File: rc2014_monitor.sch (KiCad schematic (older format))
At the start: 24 parts, among them J1 RC2014Pro, J2 Conn_01x23, SW1 SW_Coded_Octal, U1 74LS138, U2 74LS151, U3 74HCT244, U4 74HCT244, U5 74HCT244

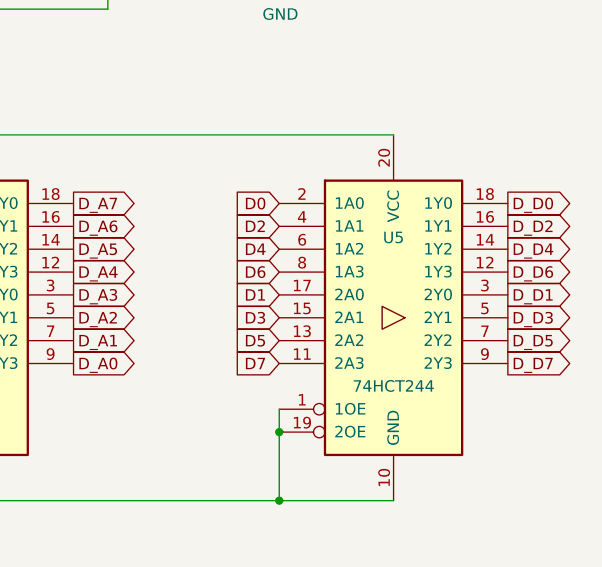
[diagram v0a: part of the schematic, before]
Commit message: started adding traces
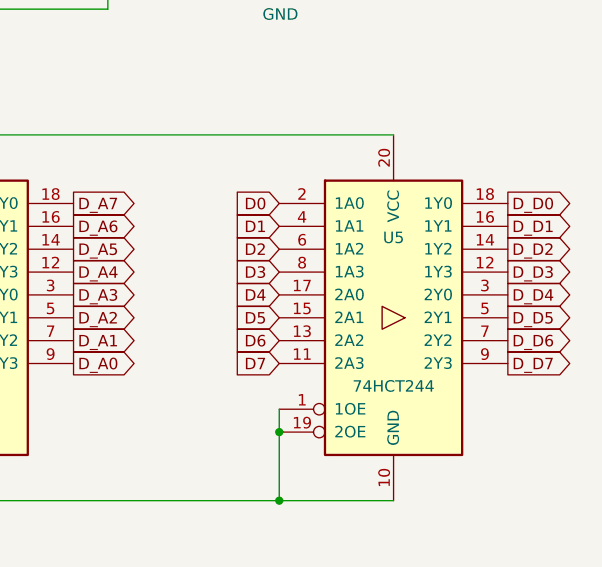
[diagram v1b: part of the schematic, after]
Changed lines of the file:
@@
 Text GLabel 8850 3650 2    50   Output ~ 0
 D_A4
-Text GLabel 9750 3850 0    50   Input ~ 0
+Text GLabel 9750 3650 0    50   Input ~ 0
 D3
+Text GLabel 9750 3550 0    50   Input ~ 0
+D2
 Text GLabel 9750 3450 0    50   Input ~ 0
-D2
-Text GLabel 9750 3750 0    50   Input ~ 0
 D1
 Text GLabel 9750 3350 0    50   Input ~ 0
@@
 Text GLabel 9750 4050 0    50   Input ~ 0
 D7
-Text GLabel 9750 3650 0    50   Input ~ 0
+Text GLabel 9750 3950 0    50   Input ~ 0
 D6
-Text GLabel 9750 3950 0    50   Input ~ 0
+Text GLabel 9750 3850 0    50   Input ~ 0
 D5
-Text GLabel 9750 3550 0    50   Input ~ 0
+Text GLabel 9750 3750 0    50   Input ~ 0
 D4
-Text GLabel 10750 3850 2    50   Output ~ 0
+Text GLabel 10750 3650 2    50   Output ~ 0
 D_D3
 Text GLabel 10750 3450 2    50   Output ~ 0
-D_D2
-Text GLabel 10750 3750 2    50   Output ~ 0
 D_D1
 Text GLabel 10750 3350 2    50   Output ~ 0
@@
 Text GLabel 10750 4050 2    50   Output ~ 0
 D_D7
-Text GLabel 10750 3650 2    50   Output ~ 0
+Text GLabel 10750 3950 2    50   Output ~ 0
 D_D6
-Text GLabel 10750 3950 2    50   Output ~ 0
+Text GLabel 10750 3850 2    50   Output ~ 0
 D_D5
-Text GLabel 10750 3550 2    50   Output ~ 0
+Text GLabel 10750 3750 2    50   Output ~ 0
 D_D4
 $Comp
@@
 NoConn ~ 1600 5700
 NoConn ~ 1600 5800
+Text GLabel 10750 3550 2    50   Output ~ 0
+D_D2
 $EndSCHEMATC

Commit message: finished traces and silkscreens
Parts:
- C1, C2, C4, C5: MouserPN (none) -> 75-1C10Z5U104M050R
- DISP0, DISP1, DISP2, DISP3, DISP4, DISP5: symbol Display_Character:TIL311 -> rc2014_monitor-rescue:TIL311-Display_Character
- LED1, LED2, LED3, LED4, LED5: MouserPN (none) -> 755-SML-H12U8TT86C
- RN1: Mouser PN 652-4607X-1LF-270 -> (none); MouserPN (none) -> 652-4607X-1LF-270
- SW1: footprint Button_Switch_SMD:Nidec_Copal_SH-7010B -> Connector_PinHeader_2.54mm:PinHeader_2x03_P2.54mm_Vertical; symbol Switch:SW_Coded_Octal -> rc2014_monitor-rescue:SW_Coded_Octal-Switch; Mouser PN 706-94HBB08RAT -> (none); MouserPN (none) -> 706-94HBB08RAT
- U1: MouserPN (none) -> 595-SN74LS138N
- U2: MouserPN (none) -> 595-SN74LS151N
- U3, U4, U5: MouserPN (none) -> 595-SN74HCT244N
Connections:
- wire segments 120 -> 118
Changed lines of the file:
@@
 $EndDescr
 $Comp
-L Display_Character:TIL311 DISP5
+L rc2014_monitor-rescue:TIL311-Display_Character DISP5
 U 1 1 5CB4BA92
 P 1950 1500
@@
 $EndComp
 $Comp
-L Display_Character:TIL311 DISP4
+L rc2014_monitor-rescue:TIL311-Display_Character DISP4
 U 1 1 5CB4CB07
 P 3500 1500
@@
 $EndComp
 $Comp
-L Display_Character:TIL311 DISP3
+L rc2014_monitor-rescue:TIL311-Display_Character DISP3
 U 1 1 5CB4D9E8
 P 5050 1500
@@
 $EndComp
 $Comp
-L Display_Character:TIL311 DISP2
+L rc2014_monitor-rescue:TIL311-Display_Character DISP2
 U 1 1 5CB570C9
 P 6600 1500
@@
 $EndComp
 $Comp
-L Display_Character:TIL311 DISP0
+L rc2014_monitor-rescue:TIL311-Display_Character DISP0
 U 1 1 5CB570D5
 P 9750 1500
@@
 F 1 "74HCT244" H 6450 3550 50  0000 C CNN
 F 2 "Package_DIP:DIP-20_W7.62mm_Socket_LongPads" H 6450 3850 50  0001 C CNN
-F 3 "https://assets.nexperia.com/documents/data-sheet/74HC_HCT244.pdf" H 6450 3850 50  0001 C CNN
+F 3 "http://www.ti.com/lit/ds/symlink/sn74hct244.pdf" H 6450 3850 50  0001 C CNN
+F 4 "595-SN74HCT244N" H 0   0   50  0001 C CNN "MouserPN"
 	1    6450 3850
 	1    0    0    -1
@@
 F 1 "74HCT244" H 8350 3550 50  0000 C CNN
 F 2 "Package_DIP:DIP-20_W7.62mm_Socket_LongPads" H 8350 3850 50  0001 C CNN
-F 3 "https://assets.nexperia.com/documents/data-sheet/74HC_HCT244.pdf" H 8350 3850 50  0001 C CNN
+F 3 "http://www.ti.com/lit/ds/symlink/sn74hct244.pdf" H 8350 3850 50  0001 C CNN
+F 4 "595-SN74HCT244N" H 0   0   50  0001 C CNN "MouserPN"
 	1    8350 3850
 	1    0    0    -1
@@
 F 1 "WR" H 4750 3550 50  0000 C CNN
 F 2 "LED_SMD:LED_0805_2012Metric_Pad1.15x1.40mm_HandSolder" V 4850 3500 50  0001 C CNN
-F 3 "~" V 4850 3500 50  0001 C CNN
+F 3 "https://www.mouser.com/datasheet/2/348/sml-h1(c)-e-1508182.pdf" V 4850 3500 50  0001 C CNN
+F 4 "755-SML-H12U8TT86C" H 0   0   50  0001 C CNN "MouserPN"
 	1    4850 3500
 	1    0    0    -1
@@
 F 1 "RD" H 4750 3650 50  0000 C CNN
 F 2 "LED_SMD:LED_0805_2012Metric_Pad1.15x1.40mm_HandSolder" V 4850 3600 50  0001 C CNN
-F 3 "~" V 4850 3600 50  0001 C CNN
+F 3 "https://www.mouser.com/datasheet/2/348/sml-h1(c)-e-1508182.pdf" V 4850 3600 50  0001 C CNN
+F 4 "755-SML-H12U8TT86C" H 0   0   50  0001 C CNN "MouserPN"
 	1    4850 3600
 	1    0    0    -1
@@
 F 1 "IORQ" H 4750 3750 50  0000 C CNN
 F 2 "LED_SMD:LED_0805_2012Metric_Pad1.15x1.40mm_HandSolder" V 4850 3700 50  0001 C CNN
-F 3 "~" V 4850 3700 50  0001 C CNN
+F 3 "https://www.mouser.com/datasheet/2/348/sml-h1(c)-e-1508182.pdf" V 4850 3700 50  0001 C CNN
+F 4 "755-SML-H12U8TT86C" H 0   0   50  0001 C CNN "MouserPN"
 	1    4850 3700
 	1    0    0    -1
@@
 F 1 "MREQ" H 4750 3850 50  0000 C CNN
 F 2 "LED_SMD:LED_0805_2012Metric_Pad1.15x1.40mm_HandSolder" V 4850 3800 50  0001 C CNN
-F 3 "~" V 4850 3800 50  0001 C CNN
+F 3 "https://www.mouser.com/datasheet/2/348/sml-h1(c)-e-1508182.pdf" V 4850 3800 50  0001 C CNN
+F 4 "755-SML-H12U8TT86C" H 0   0   50  0001 C CNN "MouserPN"
 	1    4850 3800
 	1    0    0    -1
@@
 F 1 "M1" H 4750 3950 50  0000 C CNN
 F 2 "LED_SMD:LED_0805_2012Metric_Pad1.15x1.40mm_HandSolder" V 4850 3900 50  0001 C CNN
-F 3 "~" V 4850 3900 50  0001 C CNN
+F 3 "https://www.mouser.com/datasheet/2/348/sml-h1(c)-e-1508182.pdf" V 4850 3900 50  0001 C CNN
+F 4 "755-SML-H12U8TT86C" H 0   0   50  0001 C CNN "MouserPN"
 	1    4850 3900
 	1    0    0    -1
@@
 F 1 "100nf" H 8515 5505 50  0000 L CNN
 F 2 "Capacitor_THT:C_Disc_D3.0mm_W1.6mm_P2.50mm" H 8438 5400 50  0001 C CNN
-F 3 "~" H 8400 5550 50  0001 C CNN
+F 3 "https://www.mouser.com/datasheet/2/427/Sprague%201C-3C%20MLC%20leaded%20capacitors%202000-1211470.pdf" H 8400 5550 50  0001 C CNN
+F 4 "75-1C10Z5U104M050R" H 0   0   50  0001 C CNN "MouserPN"
 	1    8400 5550
 	1    0    0    -1
@@
 F 1 "100nf" H 8065 5505 50  0000 L CNN
 F 2 "Capacitor_THT:C_Disc_D3.0mm_W1.6mm_P2.50mm" H 7988 5400 50  0001 C CNN
-F 3 "~" H 7950 5550 50  0001 C CNN
+F 3 "https://www.mouser.com/datasheet/2/427/Sprague%201C-3C%20MLC%20leaded%20capacitors%202000-1211470.pdf" H 7950 5550 50  0001 C CNN
+F 4 "75-1C10Z5U104M050R" H 0   0   50  0001 C CNN "MouserPN"
 	1    7950 5550
 	1    0    0    -1
@@
 F 2 "Package_DIP:DIP-16_W7.62mm_Socket_LongPads" H 4000 5950 50  0001 C CNN
 F 3 "http://www.ti.com/lit/gpn/sn74LS151" H 4000 5950 50  0001 C CNN
+F 4 "595-SN74LS151N" H 0   0   50  0001 C CNN "MouserPN"
 	1    4000 5950
 	1    0    0    -1
@@
 	1    0    0    -1
 $EndComp
-$Comp
-L Switch:SW_Coded_Octal SW?
-U 1 1 5CA7C108
-P 2400 3550
-AR Path="/5CB5AB00/5CB63856/5CA7C108" Ref="SW?"  Part="1"
-AR Path="/5CA7C108" Ref="SW1"  Part="1"
-F 0 "SW1" H 2532 4025 50  0000 C CNN
-F 1 "SW_Coded_Octal" H 2532 3934 50  0000 C CNN
-F 2 "Button_Switch_SMD:Nidec_Copal_SH-7010B" H 2375 3575 50  0001 C CNN
-F 3 "https://www.mouser.com/datasheet/2/626/DIP_Series_94H-334494.pdf" H 2375 3575 50  0001 C CNN
-F 4 "706-94HBB08RAT" H 2500 3150 50  0001 C CNN "Mouser PN"
-	1    2400 3550
-	1    0    0    -1
-$EndComp
 NoConn ~ 4500 4200
 NoConn ~ 4500 4100
@@
 F 2 "Package_DIP:DIP-16_W7.62mm_Socket_LongPads" H 4000 3800 50  0001 C CNN
 F 3 "http://www.ti.com/lit/gpn/sn74LS138" H 4000 3800 50  0001 C CNN
+F 4 "595-SN74LS138N" H 0   0   50  0001 C CNN "MouserPN"
 	1    4000 3800
 	1    0    0    -1
@@
 F 1 "100nf" H 9515 5505 50  0000 L CNN
 F 2 "Capacitor_THT:C_Disc_D3.0mm_W1.6mm_P2.50mm" H 9438 5400 50  0001 C CNN
-F 3 "~" H 9400 5550 50  0001 C CNN
+F 3 "https://www.mouser.com/datasheet/2/427/Sprague%201C-3C%20MLC%20leaded%20capacitors%202000-1211470.pdf" H 9400 5550 50  0001 C CNN
+F 4 "75-1C10Z5U104M050R" H 0   0   50  0001 C CNN "MouserPN"
 	1    9400 5550
 	1    0    0    -1
@@
 F 1 "100nf" H 10015 5505 50  0000 L CNN
 F 2 "Capacitor_THT:C_Disc_D3.0mm_W1.6mm_P2.50mm" H 9938 5400 50  0001 C CNN
-F 3 "~" H 9900 5550 50  0001 C CNN
+F 3 "https://www.mouser.com/datasheet/2/427/Sprague%201C-3C%20MLC%20leaded%20capacitors%202000-1211470.pdf" H 9900 5550 50  0001 C CNN
+F 4 "75-1C10Z5U104M050R" H 0   0   50  0001 C CNN "MouserPN"
 	1    9900 5550
 	1    0    0    -1
@@
 Wire Wire Line
 	3000 3600 3500 3600
-Connection ~ 2900 3500
 Connection ~ 4000 4500
 Connection ~ 9400 5400
@@
 Connection ~ 8200 800
 $Comp
-L Display_Character:TIL311 DISP1
+L rc2014_monitor-rescue:TIL311-Display_Character DISP1
 U 1 1 5CB570CF
 P 8100 1500
@@
 F 1 "74HCT244" H 10250 3550 50  0000 C CNN
 F 2 "Package_DIP:DIP-20_W7.62mm_Socket_LongPads" H 10250 3850 50  0001 C CNN
-F 3 "https://assets.nexperia.com/documents/data-sheet/74HC_HCT244.pdf" H 10250 3850 50  0001 C CNN
+F 3 "http://www.ti.com/lit/ds/symlink/sn74hct244.pdf" H 10250 3850 50  0001 C CNN
+F 4 "595-SN74HCT244N" H 0   0   50  0001 C CNN "MouserPN"
 	1    10250 3850
 	1    0    0    -1
@@
 Text GLabel 1350 1550 0    50   Input ~ 0
 D_A12
-Wire Wire Line
-	2900 3500 2900 3600
 Wire Wire Line
 	3500 5850 3350 5850
@@
 F 2 "Resistor_THT:R_Array_SIP7" V 5725 3800 50  0001 C CNN
 F 3 "https://www.mouser.com/datasheet/2/54/600x-776645.pdf" H 5350 3800 50  0001 C CNN
-F 4 "652-4607X-1LF-270" V 5350 3800 50  0001 C CNN "Mouser PN"
+F 4 "652-4607X-1LF-270" V 5350 3800 50  0001 C CNN "MouserPN"
 	1    5350 3800
 	0    1    1    0
 $EndComp
-Connection ~ 2900 3600
-Wire Wire Line
-	2900 3600 2900 3700
-Connection ~ 2900 3700
-Wire Wire Line
-	2900 3700 2900 6450
 Wire Wire Line
 	5650 3100 5650 3500
@@
 Text GLabel 10750 3550 2    50   Output ~ 0
 D_D2
+Wire Wire Line
+	2900 3500 2900 6450
+Connection ~ 2900 3500
+$Comp
+L rc2014_monitor-rescue:SW_Coded_Octal-Switch SW?
+U 1 1 5CA7C108
+P 2400 3550
+AR Path="/5CB5AB00/5CB63856/5CA7C108" Ref="SW?"  Part="1"
+AR Path="/5CA7C108" Ref="SW1"  Part="1"
+F 0 "SW1" H 2532 4025 50  0000 C CNN
+F 1 "SW_Coded_Octal" H 2532 3934 50  0000 C CNN
+F 2 "Connector_PinHeader_2.54mm:PinHeader_2x03_P2.54mm_Vertical" H 2375 3575 50  0001 C CNN
+F 3 "https://www.mouser.com/datasheet/2/626/DIP_Series_94H-334494.pdf" H 2375 3575 50  0001 C CNN
+F 4 "706-94HBB08RAT" H 2500 3150 50  0001 C CNN "MouserPN"
+	1    2400 3550
+	1    0    0    -1
+$EndComp
 $EndSCHEMATC

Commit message: updated boms
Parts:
- C1, C2, C4, C5: MFR (none) -> Vishay/Sprague; MPN (none) -> 1C10Z5U104M050R; SPN (none) -> 75-1C10Z5U104M050R; SPR (none) -> Mouser; SPURL (none) -> -
- DISP0, DISP1, DISP2, DISP3, DISP4, DISP5, J1, J2, SW1: MFR (none) -> -; MPN (none) -> -; SPN (none) -> -; SPR (none) -> -; SPURL (none) -> -
- LED1: value WR -> SMD Red 620nm 40mcd 2.2V; 20mA; MFR (none) -> ROHM Semiconductor; MPN (none) -> SML-H12U8TT86C; SPN (none) -> 755-SML-H12U8TT86C; SPR (none) -> Mouser; SPURL (none) -> -
- LED2: value RD -> SMD Red 620nm 40mcd 2.2V; 20mA; MFR (none) -> ROHM Semiconductor; MPN (none) -> SML-H12U8TT86C; SPN (none) -> 755-SML-H12U8TT86C; SPR (none) -> Mouser; SPURL (none) -> -
- LED3: value IORQ -> SMD Red 620nm 40mcd 2.2V; 20mA; MFR (none) -> ROHM Semiconductor; MPN (none) -> SML-H12U8TT86C; SPN (none) -> 755-SML-H12U8TT86C; SPR (none) -> Mouser; SPURL (none) -> -
- LED4: value MREQ -> SMD Red 620nm 40mcd 2.2V; 20mA; MFR (none) -> ROHM Semiconductor; MPN (none) -> SML-H12U8TT86C; SPN (none) -> 755-SML-H12U8TT86C; SPR (none) -> Mouser; SPURL (none) -> -
- LED5: value M1 -> SMD Red 620nm 40mcd 2.2V; 20mA; MFR (none) -> ROHM Semiconductor; MPN (none) -> SML-H12U8TT86C; SPN (none) -> 755-SML-H12U8TT86C; SPR (none) -> Mouser; SPURL (none) -> -
- RN1: MFR (none) -> Bourns; MPN (none) -> 4607X-101-271LF; SPN (none) -> 652-4607X-1LF-270; SPR (none) -> Mouser; SPURL (none) -> -
- U1, U2: MFR (none) -> Texas Instruments; MPN (none) -> SN74LS138N; SPN (none) -> 595-SN74LS138N; SPR (none) -> Mouser; SPURL (none) -> -
- U3, U4, U5: MFR (none) -> Texas Instruments; MPN (none) -> SN74HCT244N; SPN (none) -> 595-SN74HCT244N; SPR (none) -> Mouser; SPURL (none) -> -
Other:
- note added: "IORQ"
- note added: "M1"
- note added: "MREQ"
- note added: "RD"
- note added: "WR"

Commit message: more appropriate latch options
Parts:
- removed C1, C2, C4, C5: 100nf, Capacitor_THT:C_Disc_D3.0mm_W1.6mm_P2.50mm, symbol Device:C
- removed SW1: SW_Coded_Octal, Connector_PinHeader_2.54mm:PinHeader_2x03_P2.54mm_Vertical, symbol rc2014_monitor-rescue:SW_Coded_Octal-Switch
- removed U1: 74LS138, Package_DIP:DIP-16_W7.62mm_Socket_LongPads, symbol 74xx:74LS138
- removed U2: 74LS151, Package_DIP:DIP-16_W7.62mm_Socket_LongPads, symbol 74xx:74LS151
- added D1: Schottky Diodes & Rectifiers 40V Vr; 6A, Package_TO_SOT_SMD:TO-252-3_TabPin2, symbol Device:D_Schottky_x2_KCom_AKA
- added J3: USB_B_Micro, Connector_USB:USB_Micro-B_Amphenol_10103594-0001LF_Horizontal, symbol Connector:USB_B_Micro
- added SW1: SW_Coded_Octal-8, Button_Switch_THT:Nidec_Copal_SH-7010C, symbol Switch:SW_Coded_Octal-8
- added U1: 74HCT138, Package_DIP:DIP-16_W7.62mm_LongPads, symbol 74xx:74HCT138
- added U2: 74HCT151, Package_DIP:DIP-16_W7.62mm_LongPads, symbol 74xx:74HCT151
- added U6: 74HCT32, symbol 74xx:74HCT32
- J2: value Conn_01x23 -> Conn_01x10; footprint Connector_PinHeader_2.54mm:PinHeader_1x23_P2.54mm_Vertical -> Connector_PinHeader_2.54mm:PinHeader_1x10_P2.54mm_Vertical; symbol Connector_Generic:Conn_01x23 -> Connector_Generic:Conn_01x10
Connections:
- net labels added: IO_RD, IO_WR, M_RD, M_WR
- wire segments 118 -> 123
- no-connect marks 46 -> 36
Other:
- note added: "IO_RD\n"
- note added: "IO_WR"
- note added: "MR_RD"
- note added: "MR_WR"
- note removed: "IORQ"
- note removed: "MREQ"
- note removed: "RD"
- note removed: "WR"

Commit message: Added io_rd/wr,mem_rd/wr for latch options
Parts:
- removed J2: Conn_01x10, Connector_PinHeader_2.54mm:PinHeader_1x10_P2.54mm_Vertical, symbol Connector_Generic:Conn_01x10
- SW1: symbol Switch:SW_Coded_Octal-8 -> rc2014_monitor-rescue:SW_Coded_Octal-8-Switch
- U1: symbol 74xx:74HCT138 -> rc2014_monitor-rescue:74HCT138-74xx
- U2: symbol 74xx:74HCT151 -> rc2014_monitor-rescue:74HCT151-74xx
- U6: footprint (none) -> Package_DIP:DIP-14_W7.62mm_LongPads; symbol 74xx:74HCT32 -> rc2014_monitor-rescue:74HCT32-74xx
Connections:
- no-connect marks 36 -> 28
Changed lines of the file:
@@
-$EndComp
-$Comp
-L Connector_Generic:Conn_01x10 J?
-U 1 1 5CA62B20
-P 1400 5300
-AR Path="/5CB5AB00/5CA62B20" Ref="J?"  Part="1"
-AR Path="/5CA62B20" Ref="J2"  Part="1"
-F 0 "J2" H 1400 5950 50  0000 C CNN
-F 1 "Conn_01x10" H 1350 5850 50  0000 C CNN
-F 2 "Connector_PinHeader_2.54mm:PinHeader_1x10_P2.54mm_Vertical" H 1400 5300 50  0001 C CNN
-F 3 "~" H 1400 5300 50  0001 C CNN
-F 4 "-" H 0   -700 50  0001 C CNN "MFR"
-F 5 "-" H 0   -700 50  0001 C CNN "MPN"
-F 6 "-" H 0   -700 50  0001 C CNN "SPR"
-F 7 "-" H 0   -700 50  0001 C CNN "SPN"
-F 8 "-" H 0   -700 50  0001 C CNN "SPURL"
-	1    1400 5300
-	-1   0    0    -1
 $EndComp
 $Comp
@@
 $EndComp
 $Comp
-L power:+5V #PWR0109
-U 1 1 5CAA9BF0
-P 5950 700
-AR Path="/5CAA9BF0" Ref="#PWR0109"  Part="1"
-AR Path="/5CB63856/5CAA9BF0" Ref="#PWR?"  Part="1"
-AR Path="/5CB5AB00/5CB63856/5CAA9BF0" Ref="#PWR?"  Part="1"
-F 0 "#PWR0109" H 5950 550 50  0001 C CNN
-F 1 "+5V" H 5965 873 50  0000 C CNN
-F 2 "" H 5950 700 50  0001 C CNN
-F 3 "" H 5950 700 50  0001 C CNN
-	1    5950 700
-	1    0    0    -1
-$EndComp
-$Comp
 L power:GND #PWR0110
 U 1 1 5CAAC638
@@
 	0    1    1    0
 $EndComp
-Text GLabel 1600 4900 2    50   Output ~ 0
-GND
 Text GLabel 1000 5900 2    50   Output ~ 0
 D0
@@
 Text GLabel 1000 3800 2    50   Output ~ 0
 A10
-Text GLabel 1600 5000 2    50   Output ~ 0
-5V
 Text Notes 600  3000 0    50   ~ 0
 RC2014 Pro Bus
@@
 Text GLabel 10750 3550 2    50   Output ~ 0
 D_D2
-Wire Notes Line
-	550  2850 2050 2850
-Wire Notes Line
-	2050 2850 2050 7400
-Wire Notes Line
-	2050 7400 550  7400
-Wire Notes Line
-	550  7400 550  2850
 Wire Wire Line
 	8350 3050 10250 3050
@@
 	9650 800  9850 800
 Wire Wire Line
-	5950 700  5950 800
+	5850 700  5850 800
 Wire Wire Line
 	1350 1900 1350 2200
@@
 	6000 2200 6600 2200
 Wire Wire Line
-	5950 800  6500 800
-Wire Wire Line
 	9150 1750 9000 1750
 Wire Wire Line
@@
 	3600 800  4950 800
 Wire Wire Line
-	5150 800  5950 800
+	5150 800  5850 800
 Wire Wire Line
 	2050 800  3400 800
@@
 Connection ~ 2750 2500
 Connection ~ 4950 800
-Connection ~ 5950 800
 Connection ~ 3400 800
 Connection ~ 3350 5950
@@
 NoConn ~ 1000 5300
 NoConn ~ 1000 5400
-NoConn ~ 1600 5100
-NoConn ~ 1600 5200
-NoConn ~ 1600 5300
-NoConn ~ 1600 5400
-NoConn ~ 1600 5500
-NoConn ~ 1600 5600
-NoConn ~ 1600 5700
-NoConn ~ 1600 5800
 Text Notes 4550 3500 0    50   ~ 0
 IO_RD\n
@@
 Connection ~ 9800 5200
 $Comp
-L Switch:SW_Coded_Octal-8 SW1
+L rc2014_monitor-rescue:SW_Coded_Octal-8-Switch SW1
 U 1 1 5CBFAB4E
 P 2800 3200
@@
 Connection ~ 2250 3700
 $Comp
-L 74xx:74HCT151 U2
+L rc2014_monitor-rescue:74HCT151-74xx U2
 U 1 1 5CC642BF
 P 4000 5950
@@
 Connection ~ 4000 6950
 $Comp
-L 74xx:74HCT138 U1
+L rc2014_monitor-rescue:74HCT138-74xx U1
 U 1 1 5CC7ABA6
 P 4000 3800
@@
 IO_WR
 $Comp
-L 74xx:74HCT32 U6
+L rc2014_monitor-rescue:74HCT32-74xx U6
 U 1 1 5CDC2417
 P 5450 5400
 F 0 "U6" H 5450 5725 50  0000 C CNN
 F 1 "74HCT32" H 5450 5634 50  0000 C CNN
-F 2 "" H 5450 5400 50  0001 C CNN
+F 2 "Package_DIP:DIP-14_W7.62mm_LongPads" H 5450 5400 50  0001 C CNN
 F 3 "http://www.ti.com/lit/gpn/sn74LS32" H 5450 5400 50  0001 C CNN
 	1    5450 5400
@@
 $EndComp
 $Comp
-L 74xx:74HCT32 U6
+L rc2014_monitor-rescue:74HCT32-74xx U6
 U 2 1 5CDC49EF
 P 5450 5950
 F 0 "U6" H 5450 6275 50  0000 C CNN
 F 1 "74HCT32" H 5450 6184 50  0000 C CNN
-F 2 "" H 5450 5950 50  0001 C CNN
+F 2 "Package_DIP:DIP-14_W7.62mm_LongPads" H 5450 5950 50  0001 C CNN
 F 3 "http://www.ti.com/lit/gpn/sn74LS32" H 5450 5950 50  0001 C CNN
 	2    5450 5950
@@
 $EndComp
 $Comp
-L 74xx:74HCT32 U6
+L rc2014_monitor-rescue:74HCT32-74xx U6
 U 3 1 5CDEC76B
 P 6600 5950
 F 0 "U6" H 6600 6275 50  0000 C CNN
 F 1 "74HCT32" H 6600 6184 50  0000 C CNN
-F 2 "" H 6600 5950 50  0001 C CNN
+F 2 "Package_DIP:DIP-14_W7.62mm_LongPads" H 6600 5950 50  0001 C CNN
 F 3 "http://www.ti.com/lit/gpn/sn74LS32" H 6600 5950 50  0001 C CNN
 	3    6600 5950
@@
 $EndComp
 $Comp
-L 74xx:74HCT32 U6
+L rc2014_monitor-rescue:74HCT32-74xx U6
 U 4 1 5CDFB601
 P 6600 5400
 F 0 "U6" H 6600 5725 50  0000 C CNN
 F 1 "74HCT32" H 6600 5634 50  0000 C CNN
-F 2 "" H 6600 5400 50  0001 C CNN
+F 2 "Package_DIP:DIP-14_W7.62mm_LongPads" H 6600 5400 50  0001 C CNN
 F 3 "http://www.ti.com/lit/gpn/sn74LS32" H 6600 5400 50  0001 C CNN
 	4    6600 5400
@@
 $EndComp
 $Comp
-L 74xx:74HCT32 U6
+L rc2014_monitor-rescue:74HCT32-74xx U6
 U 5 1 5CE094FD
 P 7500 5650
 F 0 "U6" H 7730 5696 50  0000 L CNN
 F 1 "74HCT32" H 7730 5605 50  0000 L CNN
-F 2 "" H 7500 5650 50  0001 C CNN
+F 2 "Package_DIP:DIP-14_W7.62mm_LongPads" H 7500 5650 50  0001 C CNN
 F 3 "http://www.ti.com/lit/gpn/sn74LS32" H 7500 5650 50  0001 C CNN
 	5    7500 5650
@@
 M_WR
 NoConn ~ 4500 5350
+$Comp
+L power:+5V #PWR0109
+U 1 1 5CAA9BF0
+P 5850 700
+AR Path="/5CAA9BF0" Ref="#PWR0109"  Part="1"
+AR Path="/5CB63856/5CAA9BF0" Ref="#PWR?"  Part="1"
+AR Path="/5CB5AB00/5CB63856/5CAA9BF0" Ref="#PWR?"  Part="1"
+F 0 "#PWR0109" H 5850 550 50  0001 C CNN
+F 1 "+5V" H 5865 873 50  0000 C CNN
+F 2 "" H 5850 700 50  0001 C CNN
+F 3 "" H 5850 700 50  0001 C CNN
+	1    5850 700
+	1    0    0    -1
+$EndComp
+Connection ~ 5850 800
+Wire Wire Line
+	5850 800  6500 800
 $EndSCHEMATC
